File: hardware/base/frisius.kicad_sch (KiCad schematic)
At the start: 0 parts

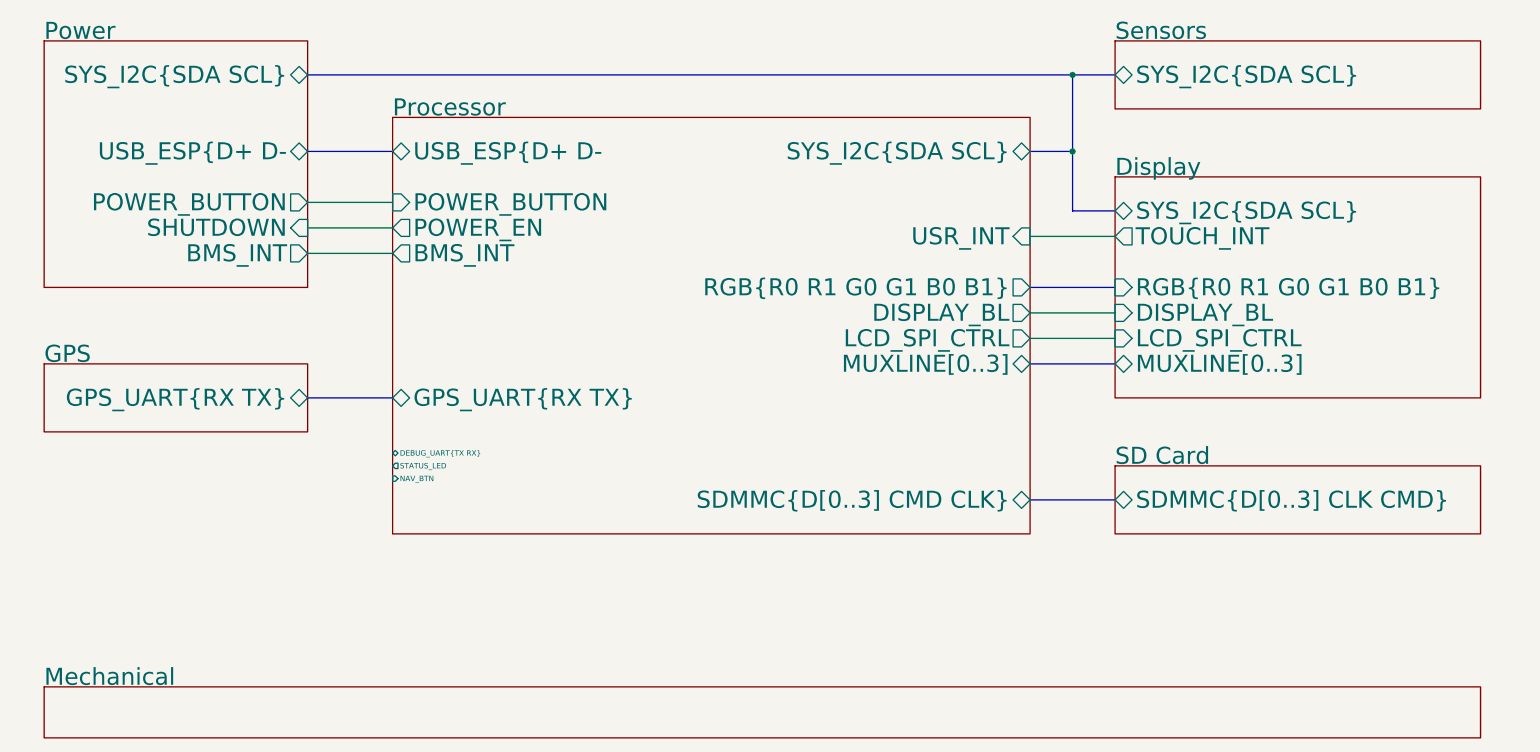
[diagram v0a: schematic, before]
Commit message: schematic complete unreviewed
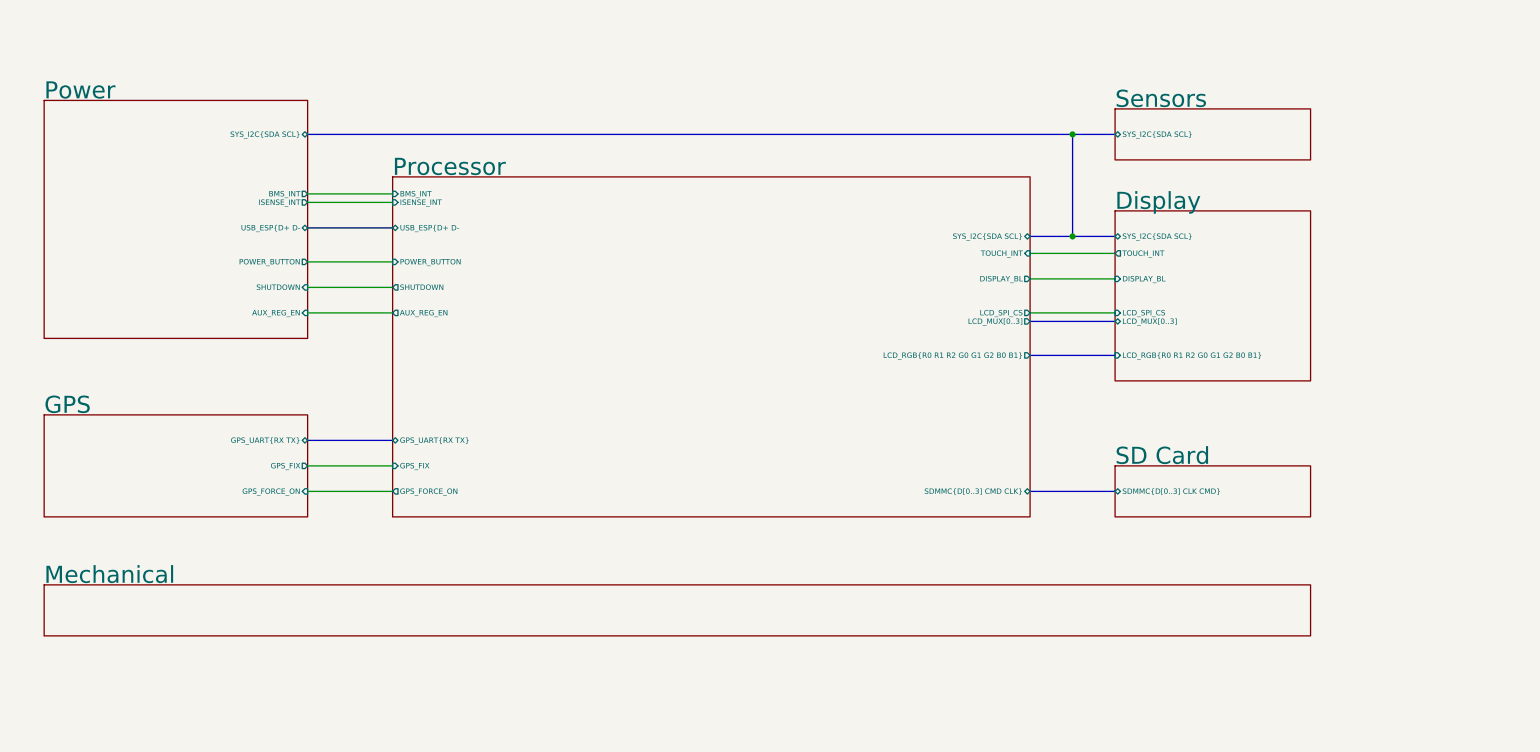
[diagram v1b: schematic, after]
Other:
- sheet Display ports: added LCD_MUX[0..3], LCD_RGB{R0 R1 R2 G0 G1 G2 B0 B1}, LCD_SPI_CS; removed LCD_SPI_CTRL, MUXLINE[0..3], RGB{R0 R1 G0 G1 B0 B1}
- sheet GPS ports: added GPS_FIX, GPS_FORCE_ON; removed none
- sheet Power ports: added AUX_REG_EN, ISENSE_INT; removed none
- sheet Processor ports: added AUX_REG_EN, GPS_FIX, GPS_FORCE_ON, ISENSE_INT, LCD_MUX[0..3], LCD_RGB{R0 R1 R2 G0 G1 G2 B0 B1}, LCD_SPI_CS, SHUTDOWN, TOUCH_INT; removed DEBUG_UART{TX RX}, LCD_SPI_CTRL, MUXLINE[0..3], NAV_BTN, POWER_EN, RGB{R0 R1 G0 G1 B0 B1}, STATUS_LED, USR_INT
